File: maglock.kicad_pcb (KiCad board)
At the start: 2 copper layers, 98 x 98 mm, 222 parts, among them J1 USB_UART, J10 Power IN, J11 12V_1, J12 12V_2, J13 5V_1, J14 5V_2, J15 5V_3, J2 I2C0_128x32, J3 I2C1, J4 SPI1, J5 I2C0_128x64, J6 USB, J7 Lock, J8 Door Open, J9 Door Close, K1 FINDER-36.11, K2 FINDER-36.11, K3 FINDER-36.11, Q1 AO3400A, Q2 AO3400A, Q3 AO3400A, Q4 AO3400A, Q5 HYG210P06LQ1D, SW1 2pin, SW2 2pin, SW3 2pin, SW4 2pin, U1 USBLC6-2SC6, U10 XL4001, U11 XL4001, U2 3V3 LDO, U3 CH340C, U4 DS18B20Z, U5 USBLC6-2SC6, U6 USBLC6-2SC6, U7 XL4001, U8 XL4001, U9 XL4001

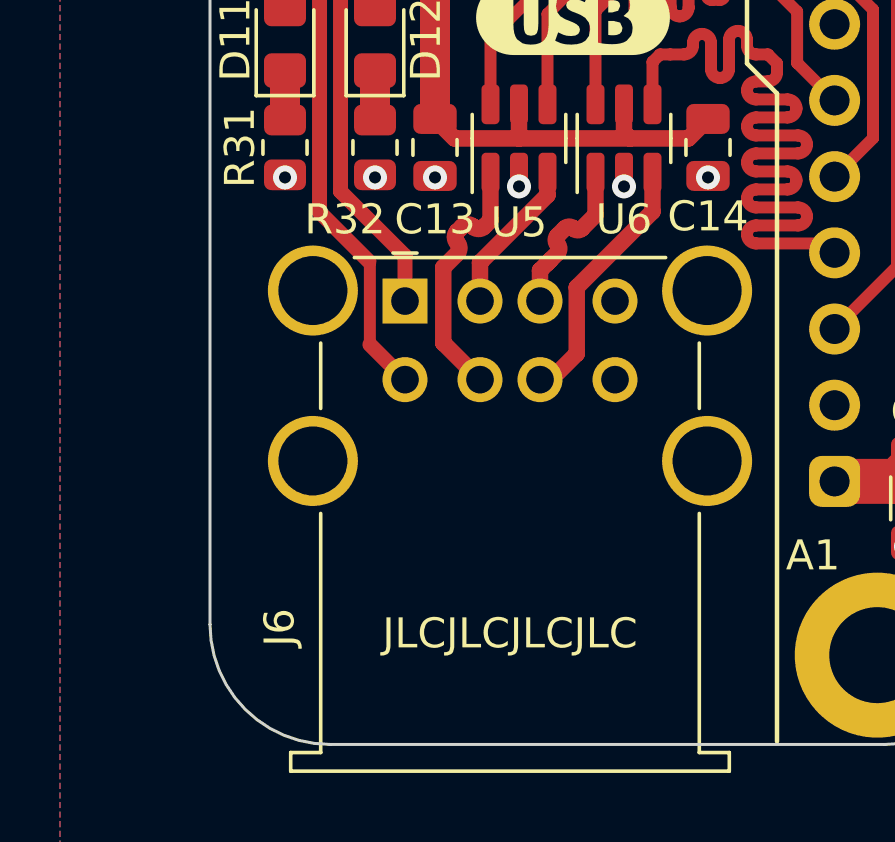
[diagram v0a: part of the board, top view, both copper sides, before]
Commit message: adding usb port 3d model
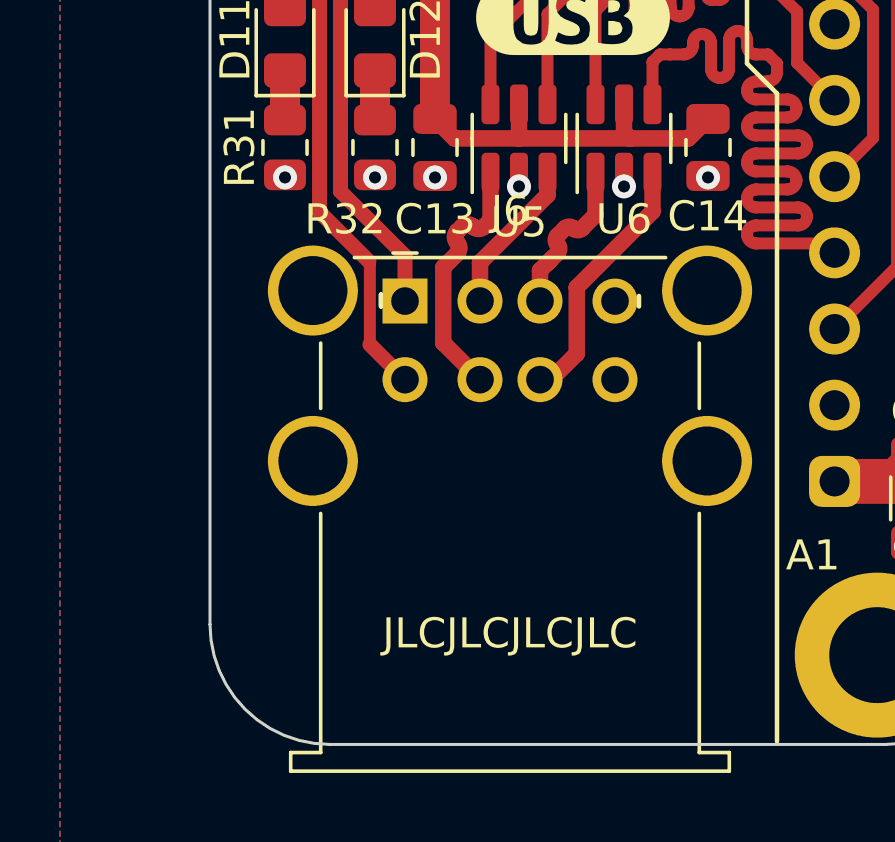
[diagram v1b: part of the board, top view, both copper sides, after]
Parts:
- J6: footprint Connector_USB:USB_A_Wuerth_61400826021_Horizontal_Stacked -> -local:USB_A_Wuerth_61400826021_Horizontal_Stacked

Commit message: ERC, DRC and BOM fixes
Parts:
- J7: value Lock -> 3pin
- J8: value Door Open -> 3pin
- J9: value Door Close -> 3pin
- K1, K2, K3: value FINDER-36.11 -> 5V Relay
- R1, R2: value 5k1 -> 4k7
- R11, R12, R13: value 100 -> 330
- R36, R37, R38, R6, R8: value 10K -> 10k

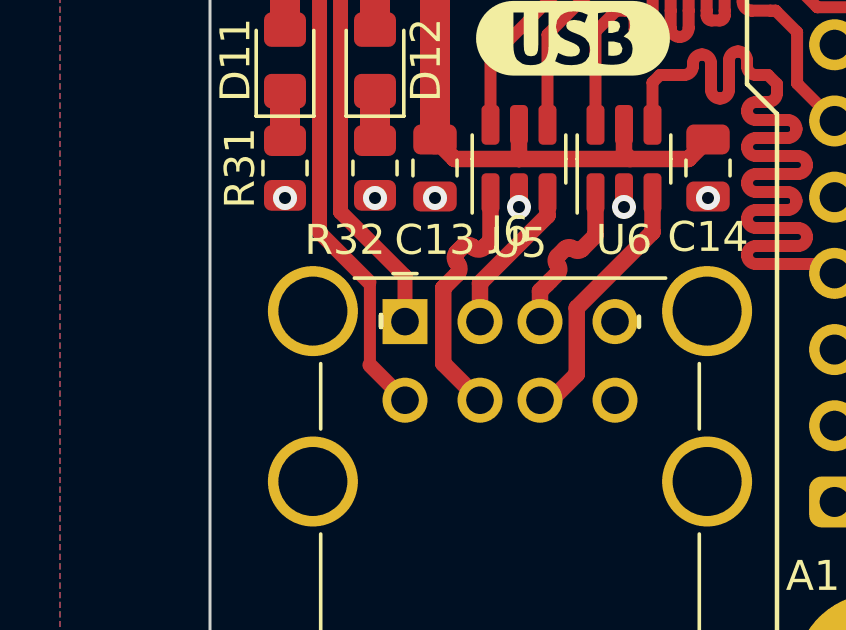
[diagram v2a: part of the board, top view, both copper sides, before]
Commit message: bom and documentation fixes
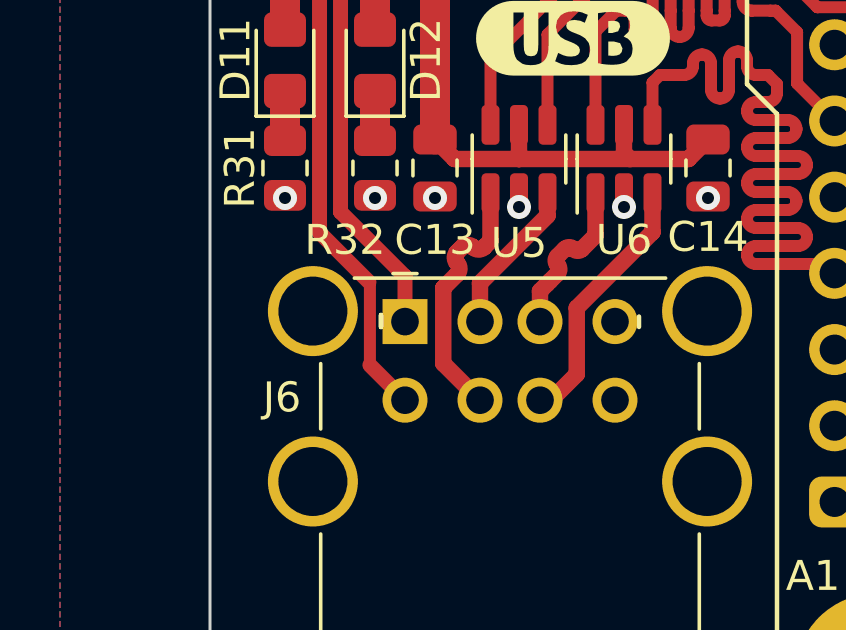
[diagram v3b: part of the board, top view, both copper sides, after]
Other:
- board text added: "Functional Overview"
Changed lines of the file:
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@@
     (attr board_only exclude_from_pos_files exclude_from_bom)
     (fp_text reference "kibuzzard-62D3EEDE" (at 0 -4.2926) (layer "F.SilkS") hide
-      (effects (font (size 0 0)))
+      (effects (font (size 0 0) (thickness 0.15)))
     )
     (fp_text value "G***" (at 0 4.2926) (layer "F.SilkS") hide
-      (effects (font (size 0 0)))
+      (effects (font (size 0 0) (thickness 0.15)))
     )
     (fp_poly (pts
@@
     (attr board_only exclude_from_pos_files exclude_from_bom)
     (fp_text reference "kibuzzard-62D2FEC2" (at 0 -4.35696) (layer "F.SilkS") hide
-      (effects (font (size 0 0)))
+      (effects (font (size 0 0) (thickness 0.15)))
     )
     (fp_text value "G***" (at 0 4.35696) (layer "F.SilkS") hide
-      (effects (font (size 0 0)))
+      (effects (font (size 0 0) (thickness 0.15)))
     )
     (fp_poly (pts
@@
     (attr board_only exclude_from_pos_files exclude_from_bom)
     (fp_text reference "kibuzzard-62D40FBB" (at 0 -4.06109 90) (layer "F.SilkS") hide
-      (effects (font (size 0 0)))
+      (effects (font (size 0 0) (thickness 0.15)))
     )
     (fp_text value "G***" (at 0 4.06109 90) (layer "F.SilkS") hide
-      (effects (font (size 0 0)))
+      (effects (font (size 0 0) (thickness 0.15)))
     )
     (fp_poly (pts
@@
     (attr board_only exclude_from_pos_files exclude_from_bom)
     (fp_text reference "kibuzzard-62D2E7EB" (at 0 -4.2926) (layer "F.SilkS") hide
-      (effects (font (size 0 0)))
+      (effects (font (size 0 0) (thickness 0.15)))
     )
     (fp_text value "G***" (at 0 4.2926) (layer "F.SilkS") hide
-      (effects (font (size 0 0)))
+      (effects (font (size 0 0) (thickness 0.15)))
     )
     (fp_poly (pts
@@
     (attr board_only exclude_from_pos_files exclude_from_bom)
     (fp_text reference "kibuzzard-62D2E07E" (at 0 -4.018955 -90) (layer "F.SilkS") hide
-      (effects (font (size 0 0)))
+      (effects (font (size 0 0) (thickness 0.15)))
     )
     (fp_text value "G***" (at 0 4.018955 -90) (layer "F.SilkS") hide
-      (effects (font (size 0 0)))
+      (effects (font (size 0 0) (thickness 0.15)))
     )
     (fp_poly (pts
@@
     (attr board_only exclude_from_pos_files exclude_from_bom)
     (fp_text reference "kibuzzard-62D3EEF7" (at 0 -4.2926) (layer "F.SilkS") hide
-      (effects (font (size 0 0)))
+      (effects (font (size 0 0) (thickness 0.15)))
     )
     (fp_text value "G***" (at 0 4.2926) (layer "F.SilkS") hide
-      (effects (font (size 0 0)))
+      (effects (font (size 0 0) (thickness 0.15)))
     )
     (fp_poly (pts
@@
     (property "Sheetname" "_USB_PORTS")
     (attr through_hole)
-    (fp_text reference "J6" (at 3.5 -3) (layer "F.SilkS")
+    (fp_text reference "J6" (at -4.1 2.53) (layer "F.SilkS")
       (effects (font (size 1 1) (thickness 0.15)))
     )
@@
     (effects (font (size 3 3) (thickness 0.75)))
   )
+  (gr_text "Functional Overview" (at 15 20) (layer "User.2")
+    (effects (font (size 6 6) (thickness 1.5)) (justify left))
+  )
   (gr_text "Relay\nOutputs" (at 184.2 77.7) (layer "User.2")
     (effects (font (size 3 3) (thickness 0.75)))
@@
     (pts (xy 131 150) (xy 131 131))
     (height 8)
-    (gr_text "19.00" (at 135.5 140.5 90) (layer "User.8")
+    (gr_text "19" (at 135.5 140.5 90) (layer "User.8")
       (effects (font (size 3 3) (thickness 0.5)))
     )
-    (format (units 3) (units_format 0) (precision 2))
+    (format (units 2) (units_format 0) (precision 2) suppress_zeroes)
     (style (thickness 0.15) (arrow_length 1.27) (text_position_mode 0) (extension_height 0.58642) (extension_offset 0.5) keep_text_aligned)
   )
@@
     (pts (xy 109 150) (xy 109 52))
     (height -14)
-    (gr_text "98.00" (at 91.5 101 90) (layer "User.8")
+    (gr_text "98" (at 91.5 101 90) (layer "User.8")
       (effects (font (size 3 3) (thickness 0.5)))
     )
-    (format (units 3) (units_format 0) (precision 2))
+    (format (units 2) (units_format 0) (precision 2) suppress_zeroes)
     (style (thickness 0.15) (arrow_length 1.27) (text_position_mode 0) (extension_height 0.58642) (extension_offset 0.5) keep_text_aligned)
   )
@@
     (pts (xy 130 146) (xy 105 146))
     (height -24)
-    (gr_text "25.00" (at 117.5 166.5) (layer "User.8")
+    (gr_text "25" (at 117.5 166.5) (layer "User.8")
       (effects (font (size 3 3) (thickness 0.5)))
     )
-    (format (units 3) (units_format 0) (precision 2))
+    (format (units 2) (units_format 0) (precision 2) suppress_zeroes)
     (style (thickness 0.15) (arrow_length 1.27) (text_position_mode 0) (extension_height 0.58642) (extension_offset 0.5) keep_text_aligned)
   )
@@
     (pts (xy 203 56) (xy 105 56))
     (height 16)
-    (gr_text "98.00" (at 154 36.5) (layer "User.8")
+    (gr_text "98" (at 154 36.5) (layer "User.8")
       (effects (font (size 3 3) (thickness 0.5)))
     )
-    (format (units 3) (units_format 0) (precision 2))
+    (format (units 2) (units_format 0) (precision 2) suppress_zeroes)
     (style (thickness 0.15) (arrow_length 1.27) (text_position_mode 0) (extension_height 0.58642) (extension_offset 0.5) keep_text_aligned)
   )
@@
     (pts (xy 157 146) (xy 130 146))
     (height -24)
-    (gr_text "27.00" (at 143.5 166.5) (layer "User.8")
+    (gr_text "27" (at 143.5 166.5) (layer "User.8")
       (effects (font (size 3 3) (thickness 0.5)))
     )
-    (format (units 3) (units_format 0) (precision 2))
+    (format (units 2) (units_format 0) (precision 2) suppress_zeroes)
     (style (thickness 0.15) (arrow_length 1.27) (text_position_mode 0) (extension_height 0.58642) (extension_offset 0.5) keep_text_aligned)
   )
@@
       (effects (font (size 3 3) (thickness 0.5)))
     )
-    (format (units 3) (units_format 0) (precision 2) suppress_zeroes)
+    (format (units 2) (units_format 0) (precision 2) suppress_zeroes)
     (style (thickness 0.15) (arrow_length 1.27) (text_position_mode 2) (extension_height 0.58642) (extension_offset 0.5) keep_text_aligned)
   )
@@
       (effects (font (size 3 3) (thickness 0.5)))
     )
-    (format (units 3) (units_format 0) (precision 2) suppress_zeroes)
+    (format (units 2) (units_format 0) (precision 2) suppress_zeroes)
     (style (thickness 0.15) (arrow_length 1.27) (text_position_mode 0) (extension_height 0.58642) (extension_offset 0.5) keep_text_aligned)
   )
@@
       (effects (font (size 3 3) (thickness 0.5)))
     )
-    (format (units 3) (units_format 0) (precision 2) suppress_zeroes)
+    (format (units 2) (units_format 0) (precision 2) suppress_zeroes)
     (style (thickness 0.15) (arrow_length 1.27) (text_position_mode 0) (extension_height 0.58642) (extension_offset 0.5) keep_text_aligned)
   )
@@
       (effects (font (size 3 3) (thickness 0.5)))
     )
-    (format (units 3) (units_format 0) (precision 2) suppress_zeroes)
+    (format (units 2) (units_format 0) (precision 2) suppress_zeroes)
     (style (thickness 0.15) (arrow_length 1.27) (text_position_mode 0) (extension_height 0.58642) (extension_offset 0.5) keep_text_aligned)
   )
@@
       (effects (font (size 3 3) (thickness 0.5)))
     )
-    (format (units 3) (units_format 0) (precision 2) suppress_zeroes)
+    (format (units 2) (units_format 0) (precision 2) suppress_zeroes)
     (style (thickness 0.15) (arrow_length 1.27) (text_position_mode 0) (extension_height 0.58642) (extension_offset 0.5) keep_text_aligned)
   )
@@
       (effects (font (size 3 3) (thickness 0.5)))
     )
-    (format (units 3) (units_format 0) (precision 2) suppress_zeroes)
+    (format (units 2) (units_format 0) (precision 2) suppress_zeroes)
     (style (thickness 0.15) (arrow_length 1.27) (text_position_mode 0) (extension_height 0.58642) (extension_offset 0.5) keep_text_aligned)
   )
@@
       (effects (font (size 3 3) (thickness 0.5)))
     )
-    (format (units 3) (units_format 0) (precision 2) suppress_zeroes)
+    (format (units 2) (units_format 0) (precision 2) suppress_zeroes)
     (style (thickness 0.15) (arrow_length 1.27) (text_position_mode 0) (extension_height 0.58642) (extension_offset 0.5) keep_text_aligned)
   )
@@
       (effects (font (size 3 3) (thickness 0.5)))
     )
-    (format (units 3) (units_format 0) (precision 2) suppress_zeroes)
+    (format (units 2) (units_format 0) (precision 2) suppress_zeroes)
     (style (thickness 0.15) (arrow_length 1.27) (text_position_mode 0) (extension_height 0.58642) (extension_offset 0.5) keep_text_aligned)
   )
